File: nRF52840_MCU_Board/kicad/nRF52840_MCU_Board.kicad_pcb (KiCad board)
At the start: 2 copper layers, 45 x 45 mm, 33 parts, among them J1 CONN_COAXIAL, U1 nRF52840, X1 XTAL_32MHZ, X2 XTAL_32KHZ

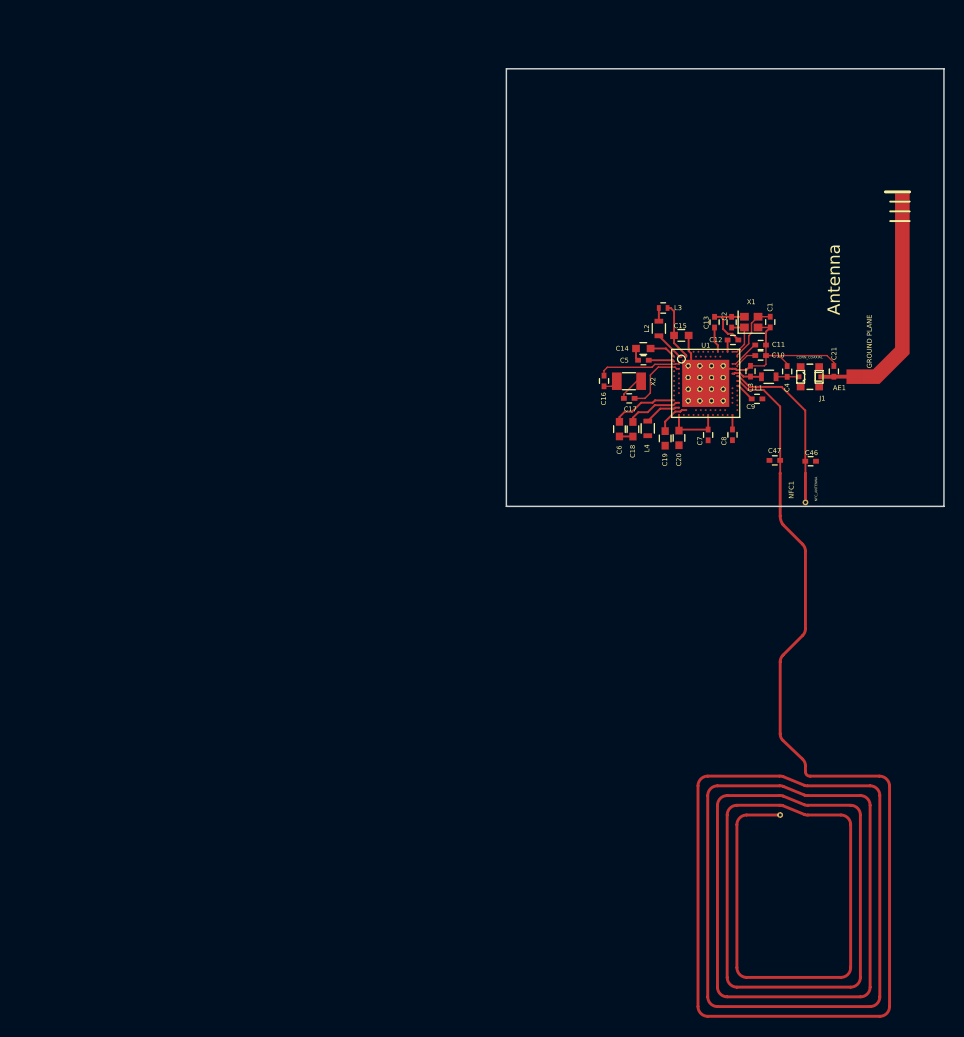
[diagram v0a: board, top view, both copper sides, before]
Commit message: Update KiCAD Project nRF52840_MCU_Board
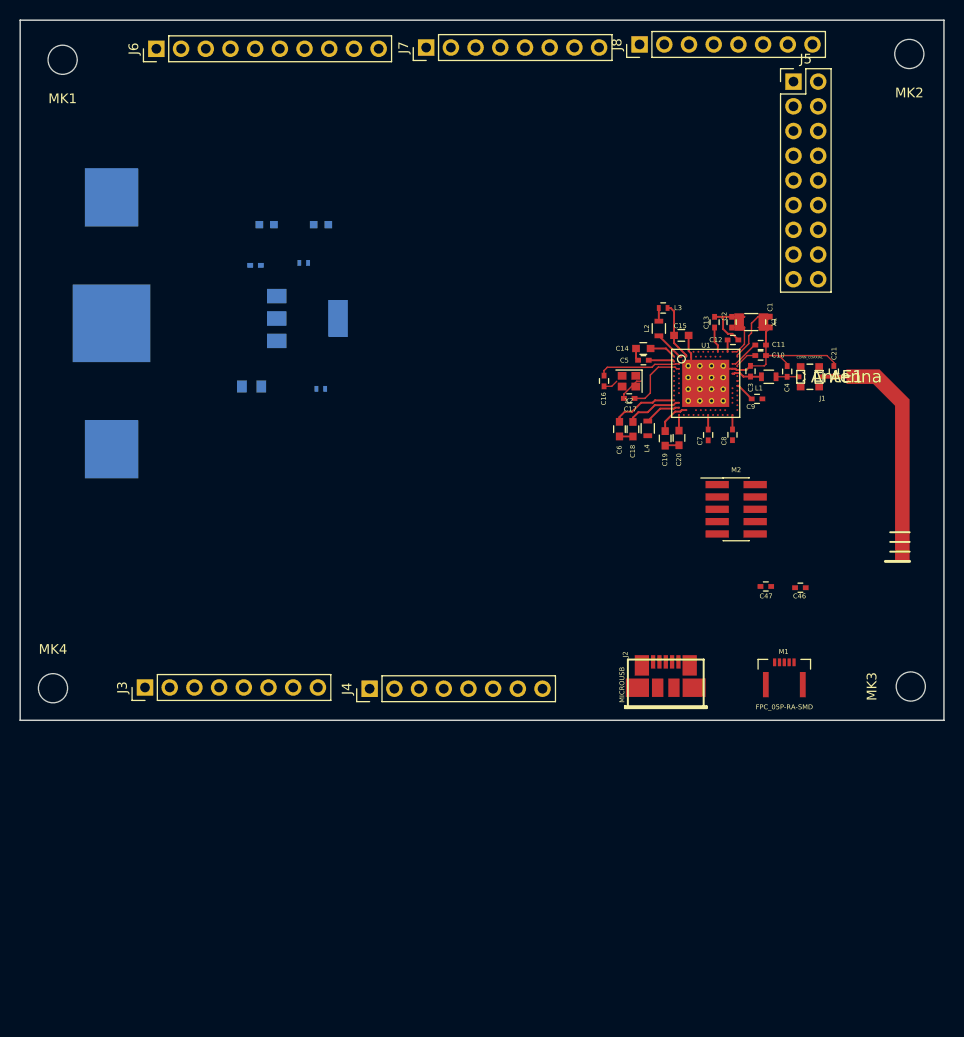
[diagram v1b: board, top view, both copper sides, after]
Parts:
- removed NFC1: NFC_ANTENNA, Nordic_misc:Nordic_misc-NFC_ANT
- added BATT1: CR2032, Nordic_misc:keystone_3003, B.Cu at (39.4, 91.2)
- added C22: 100nF, Capacitors_SMD:C_0402, B.Cu at (54.2, 85.2)
- added C23: 10uF, Capacitors_SMD:C_0603, B.Cu at (55.3, 81.0)
- added C24: 10uF, Capacitors_SMD:C_0603, B.Cu at (60.9, 81.0)
- added C25: 100uF, Capacitors_SMD:C_0805, B.Cu at (53.8, 97.7)
- added J2: MICROUSB, Nordic_misc:conn_usb_B_micro_smd, F.Cu at (96.4, 128.7)
- added J3: Power, Pin_Headers:Pin_Header_Straight_1x08_Pitch2.54mm, F.Cu at (42.8, 128.6)
- added J4: Analog, Pin_Headers:Pin_Header_Straight_1x08_Pitch2.54mm, F.Cu at (65.9, 128.8)
- added J5: Digital3, Pin_Headers:Pin_Header_Straight_2x09_Pitch2.54mm, F.Cu at (109.5, 66.3)
- added J6: Digital0, Pin_Headers:Pin_Header_Straight_1x10_Pitch2.54mm, F.Cu at (44.0, 62.9)
- added J7: Digital1, Pin_Headers:Pin_Header_Straight_1x08_Pitch2.54mm, F.Cu at (71.8, 62.8)
- added J8: Digital2, Pin_Headers:Pin_Header_Straight_1x08_Pitch2.54mm, F.Cu at (93.7, 62.5)
- added M1: FPC_05P-RA-SMD, Nordic_misc:Nordic_misc-FPC_05P-RA-SMD, F.Cu at (108.6, 127.6)
- added M2: DEBUG_CONNECTOR, Nordic_misc:Pin_Header_Straight_2x05_Pitch1.27mm_SMD, F.Cu at (103.6, 110.3)
- added MK1: Mounting_Hole, Nordic_misc:MountingHole_3mm, F.Cu at (34.4, 64.1)
- added MK2: Mounting_Hole, Nordic_misc:MountingHole_3mm, F.Cu at (121.4, 63.5)
- added MK3: Mounting_Hole, Nordic_misc:MountingHole_3mm, F.Cu at (121.6, 128.5)
- added MK4: Mounting_Hole, Nordic_misc:MountingHole_3mm, F.Cu at (33.4, 128.7)
- added R1: 0, Resistors_SMD:R_0402, B.Cu at (59.2, 85.0)
- added R2: 0, Resistors_SMD:R_0402, B.Cu at (60.9, 97.9)
- added U2: TLV1117, TO_SOT_Packages_SMD:SOT-223-3Lead_TabPin2, B.Cu at (59.5, 90.7)
- AE1: footprint Nordic_misc:Nordic_misc-QWMP_BEND_LEFT_+0 -> Nordic_misc:Nordic_misc-QWMP_BEND_RIGHT_+0
- X1: value XTAL_32MHZ -> XTAL_32KHZ; footprint Nordic_nRF:Crystal_SMD_2016-4pin_2.0x1.6mm -> Nordic_nRF:Crystal_SMD_3215-2pin_3.2x1.5mm
- X2: value XTAL_32KHZ -> XTAL_32MHZ; footprint Nordic_nRF:Crystal_SMD_3215-2pin_3.2x1.5mm -> Nordic_nRF:Crystal_SMD_2016-4pin_2.0x1.6mm
- moved C46 13.0 mm to (110.2, 118.4), turned to 0 degrees
- moved C47 13.0 mm to (106.7, 118.2), turned to 0 degrees
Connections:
- C46 pad 1: GND -> /nRF52840/NFC2
- C46 pad 2: /NFC2 -> GND
- C47 pad 1: /NFC1 -> GND
- C47 pad 2: GND -> /nRF52840/NFC1
- U1 pad AA24: (no net) -> Net-(M2-Pad4)
- U1 pad AC13: (no net) -> /nRF52840/P0.18/RESET
- U1 pad AC24: (no net) -> Net-(M2-Pad2)
- U1 pad AD22: (no net) -> /nRF52840/P1.00
- U1 pad AD4: (no net) -> /D-
- U1 pad AD6: (no net) -> /D+
- U1 pad J24: /NFC2 -> /nRF52840/NFC2
- U1 pad L24: /NFC1 -> /nRF52840/NFC1
- X1 pad 1: Net-(C2-Pad2) -> Net-(C16-Pad2)
- X1 pad 2: GND -> Net-(C17-Pad2)
- X2 pad 1: Net-(C16-Pad2) -> Net-(C2-Pad2)
- X2 pad 2: Net-(C17-Pad2) -> GND
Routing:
- net /NFC2: track 14.9 -> 0.00 mm
- net /NFC1: track 12.4 -> 0.00 mm
- net +3V3: track 18.6 -> 15.7 mm
- net GND: track 37.5 -> 39.1 mm
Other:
- board size 45 x 45 mm -> 95 x 72 mm
